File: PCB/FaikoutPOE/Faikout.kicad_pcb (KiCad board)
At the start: 2 copper layers, 58 x 36 mm, 83 parts, among them J1 RJ45_LED, J2 S21, J5 Reset, J7 TC2030-USB-NL-DS, M3 Ag97012-FL, P1 Square, Q1 BSS138PS, U1 KSZ8851SNL, U2 ESP32-S3-MINI-1, U3 TCMT1100, U4 TPS62933, U5 TCMT1100, Y1 Crystal_GND24

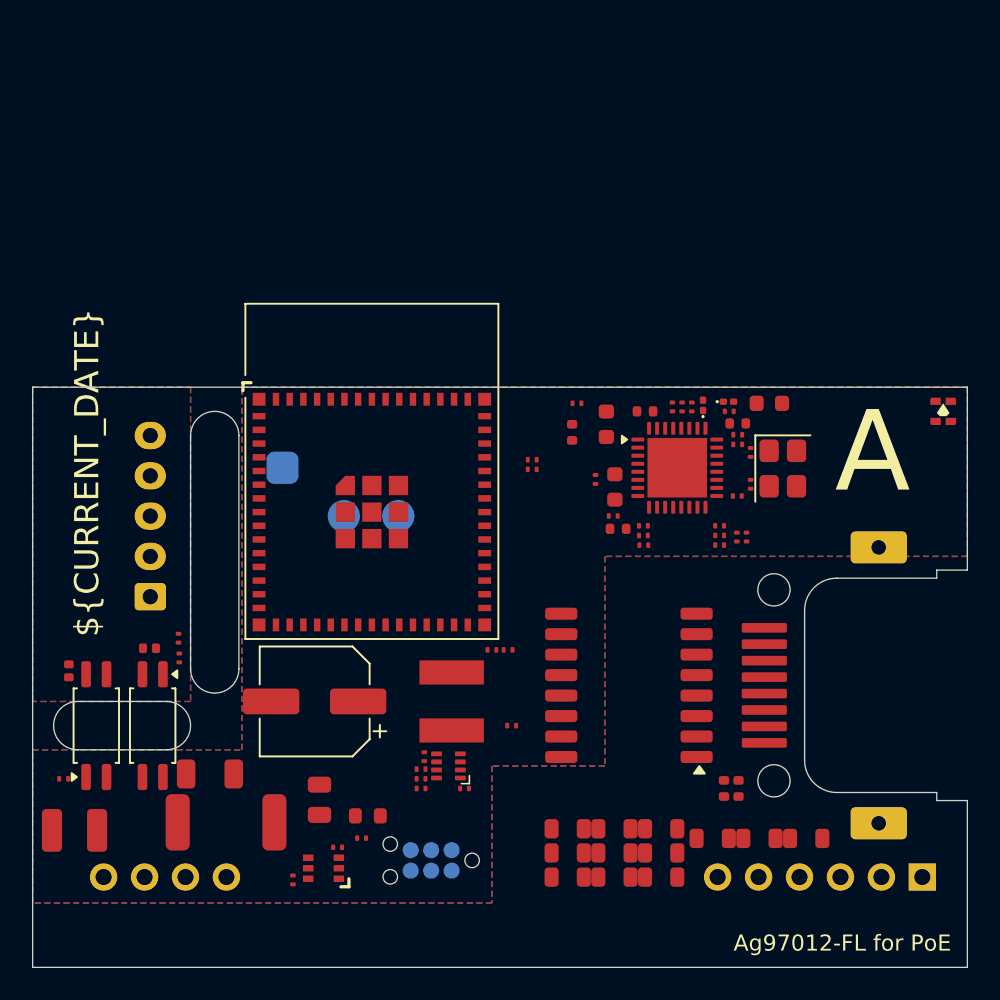
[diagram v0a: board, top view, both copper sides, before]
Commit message: Tidy models
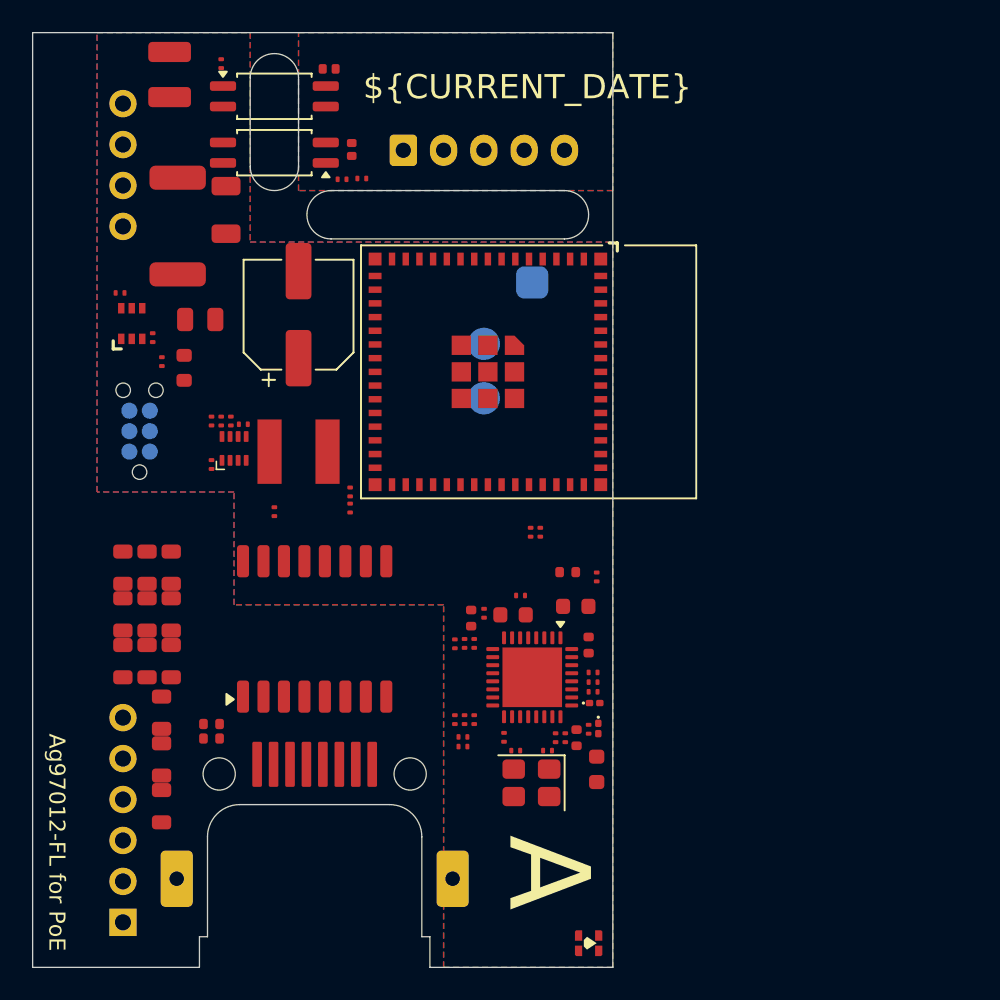
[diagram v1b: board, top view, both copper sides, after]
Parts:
- moved M3 49.7 mm to (105.6, 97.2), turned to 180 degrees
- moved F3 47.3 mm to (108.5, 44.6), turned to -90 degrees
- moved R5 45.4 mm to (111.7, 43.9), turned to -90 degrees
- moved D3 40.7 mm to (118.4, 44.2), turned to 180 degrees
- moved U3 40.6 mm to (115.0, 46.0), turned to 0 degrees
- moved L12 40.0 mm to (108.0, 90.0), turned to -90 degrees
- moved D4 39.7 mm to (134.5, 98.5), turned to 180 degrees
- moved R22 38.0 mm to (105.4, 58.1), turned to 180 degrees
- moved L11 37.4 mm to (108.0, 87.1), turned to -90 degrees
- moved R20 37.1 mm to (109.0, 54.0), turned to -90 degrees
- moved J1 37.0 mm to (117.5, 94.5), turned to 0 degrees
- moved U5 36.3 mm to (115.0, 49.5), turned to 180 degrees
- moved L9 36.0 mm to (105.6, 81.0), turned to -90 degrees
- moved Q1 35.8 mm to (106.2, 60.0), turned to 90 degrees
- moved L10 35.1 mm to (108.0, 84.2), turned to -90 degrees
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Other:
- board size 58 x 36 mm -> 36 x 58 mm
